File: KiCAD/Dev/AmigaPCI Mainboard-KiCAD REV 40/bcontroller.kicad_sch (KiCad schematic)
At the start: 32 parts, among them CN409 SPI, J901 IDE MODES, U111 74LVC16646, U112 74LVC16646, U409 ICE40HX4K-TQ144, U409F1 W25X20CLSN

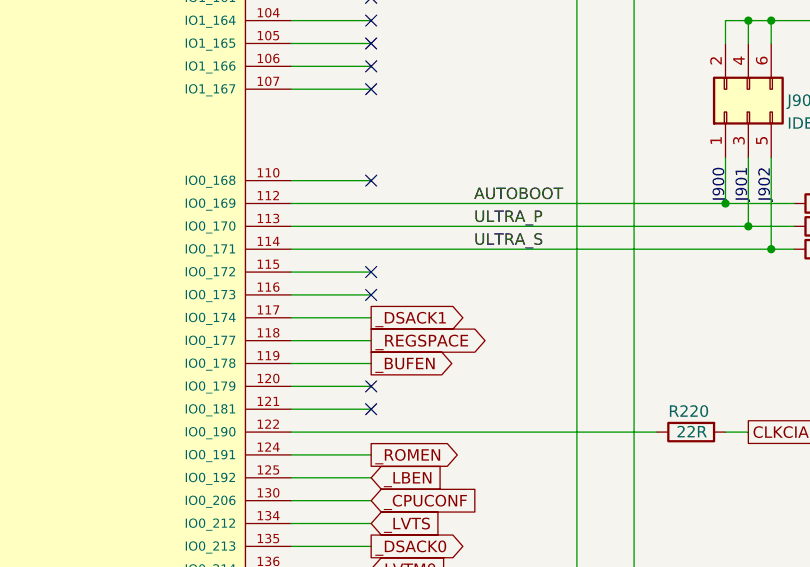
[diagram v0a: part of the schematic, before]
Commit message: AmigaPCI Mainboard REV 4.0 Routing
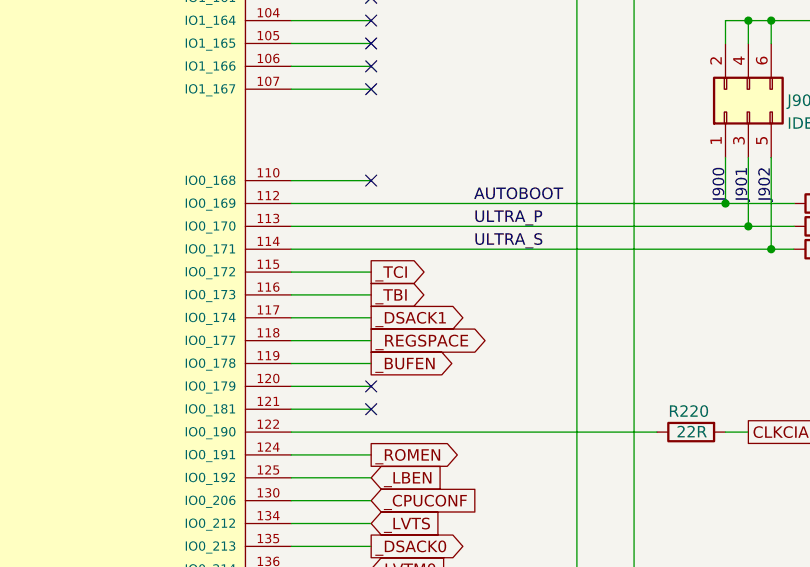
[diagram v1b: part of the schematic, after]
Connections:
- net _TCI: now reaches U409.115 (IO0_172)
- net _TBI: now reaches U409.116 (IO0_173)
- no-connect marks 28 -> 26
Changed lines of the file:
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@@
 	(title_block
 		(title "AMIGA PCI")
-		(date "2024-07-17")
+		(date "2024-07-31")
 		(rev "4.0")
 	)
@@
 	)
 	(no_connect
-		(at 147.32 185.42)
-	)
-	(no_connect
 		(at 147.32 162.56)
 	)
@@
 	)
 	(no_connect
-		(at 147.32 182.88)
-	)
-	(no_connect
 		(at 147.32 142.24)
 	)
@@
 		)
 	)
+	(global_label "_TCI"
+		(shape output)
+		(at 147.32 182.88 0)
+		(fields_autoplaced yes)
+		(effects
+			(font
+				(size 1.27 1.27)
+			)
+			(justify left)
+		)
+		(property "Intersheetrefs" "${INTERSHEET_REFS}"
+			(at 154.1152 182.88 0)
+			(effects
+				(font
+					(size 1.27 1.27)
+				)
+				(justify left)
+			)
+		)
+	)
 	(global_label "PIO_S0"
 		(shape output)
@@
 			(effects
 				(font
+					(size 1.27 1.27)
+				)
+				(justify left)
+			)
+		)
+	)
+	(global_label "_TBI"
+		(shape output)
+		(at 147.32 185.42 0)
+		(fields_autoplaced yes)
+		(effects
+			(font
+				(size 1.27 1.27)
+			)
+			(justify left)
+		)
+		(property "Intersheetrefs" "${INTERSHEET_REFS}"
+			(at 154.1152 185.42 0)
+			(effects
+				(font
